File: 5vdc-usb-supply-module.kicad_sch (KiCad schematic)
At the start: 6 parts

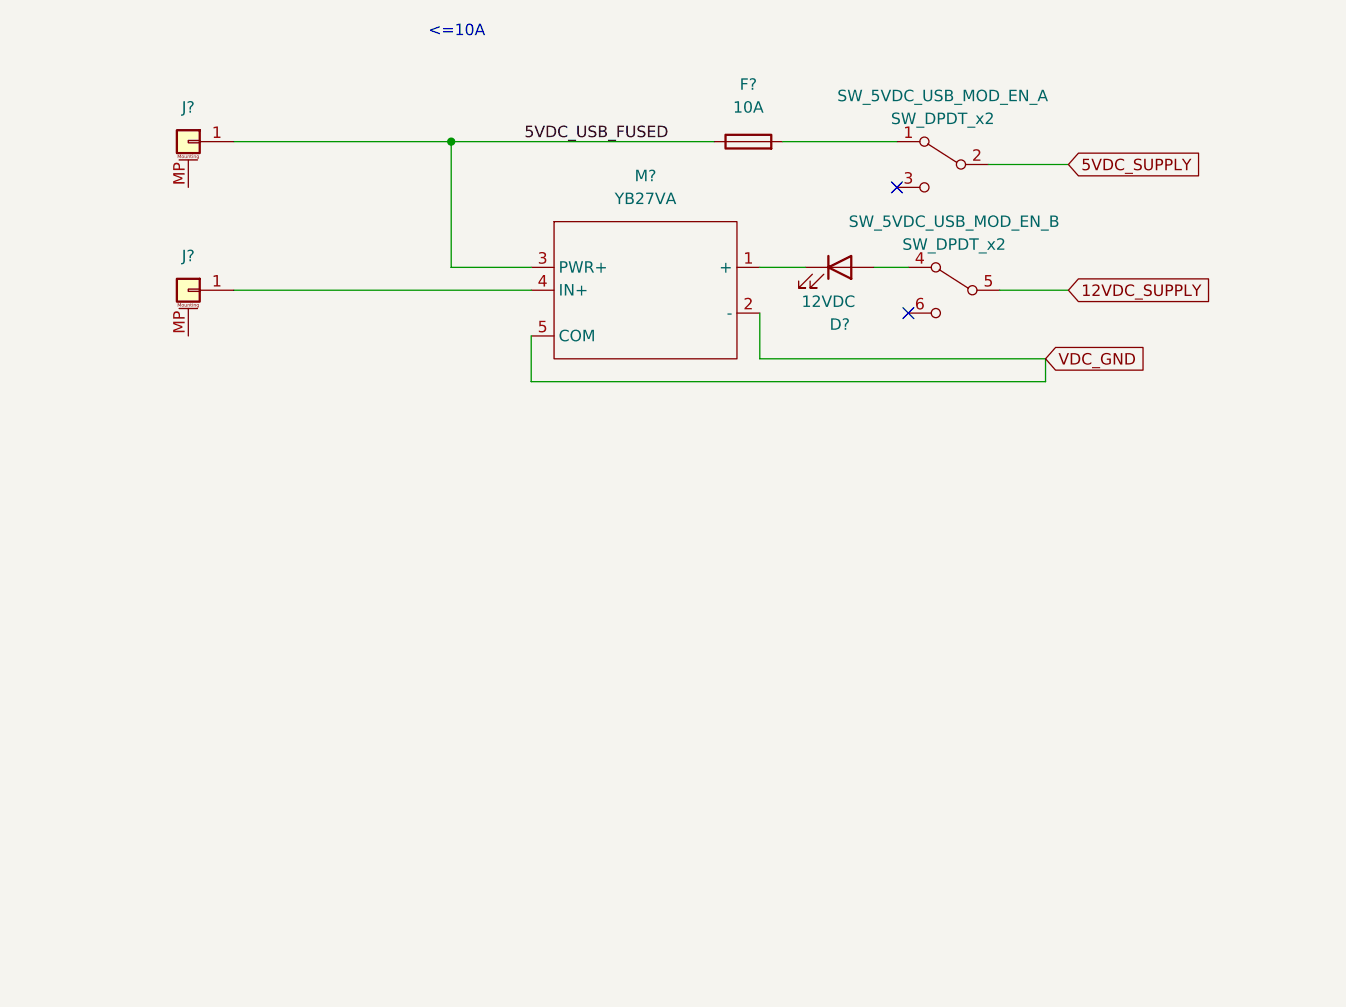
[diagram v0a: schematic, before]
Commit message: Bunch more changes
Blah blah
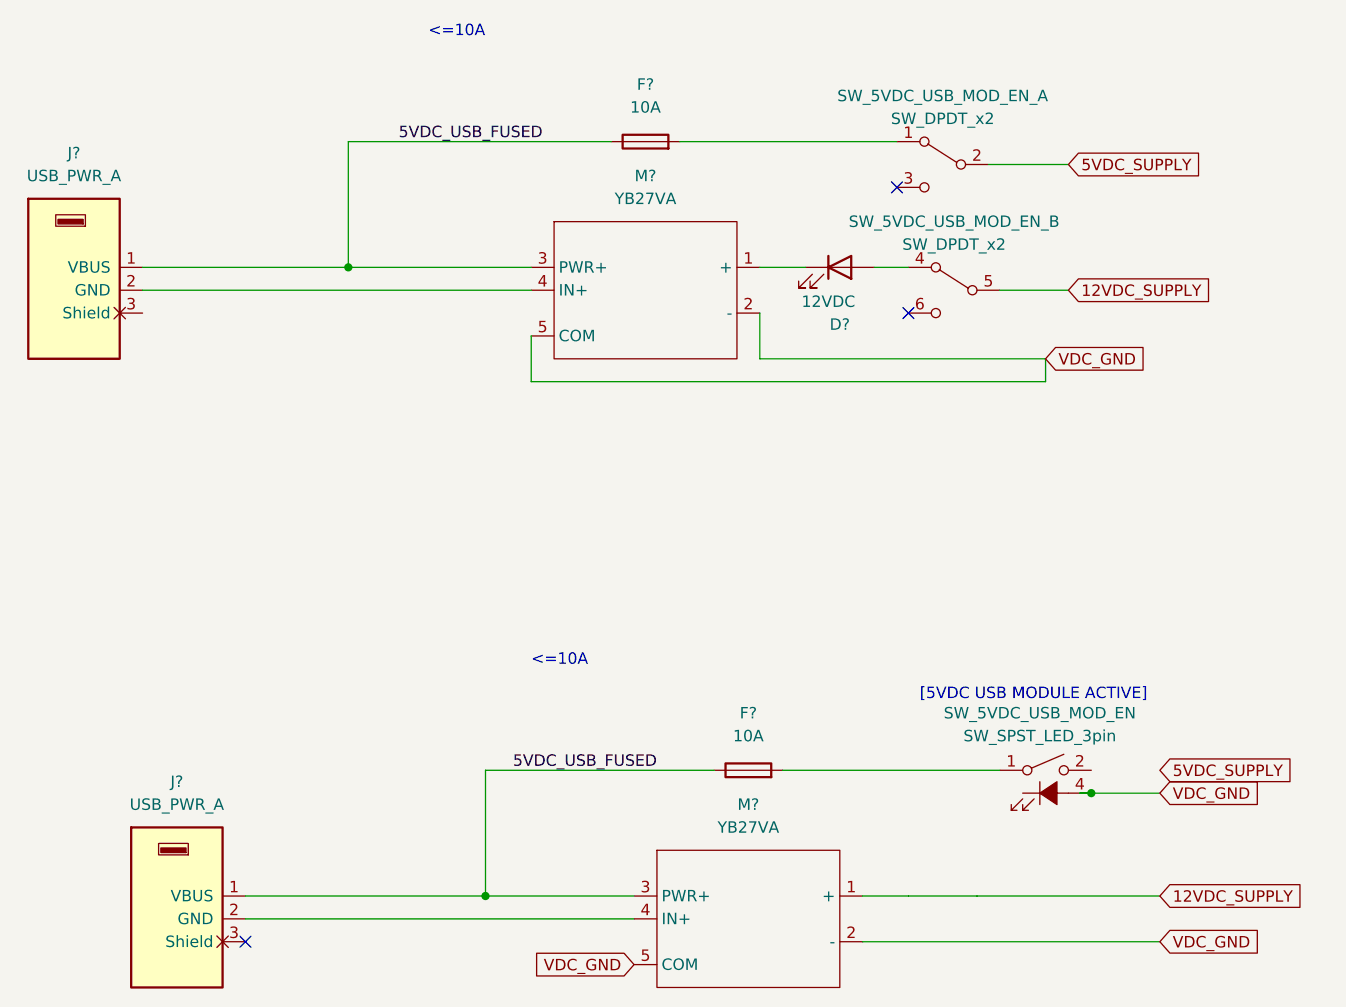
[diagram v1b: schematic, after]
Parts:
- removed J? (x2): Conn_01x01_MountingPin, symbol Connector_Generic_MountingPin:Conn_01x01_MountingPin
- added F?: 10A, symbol Device:Fuse
- added M?: YB27VA, symbol bvm-library:5_Pin_Meter_With_Ext_Shunt
- added SW_5VDC_USB_MOD_EN: SW_SPST_LED_3pin, symbol bvm-library:SW_SPST_LED_3pin
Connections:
- net 12VDC_SUPPLY: now also M?.1 (+)
- net 5VDC_USB_FUSED: now also F?.1, M?.3 (PWR+)
- net VDC_GND: now also M?.2 (-), M?.5 (COM), SW_5VDC_USB_MOD_EN.4 (A)
- net GND: now reaches M?.4 (IN+)
- net GND: now also M?.4 (IN+)
- new net: F?.2, SW_5VDC_USB_MOD_EN.1
- no-connect marks 2 -> 3
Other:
- note added: "[5VDC USB MODULE ACTIVE]"
- title: (none) -> Mr. Powers
- moved on the sheet: F?
